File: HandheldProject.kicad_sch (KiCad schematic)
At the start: 16 parts

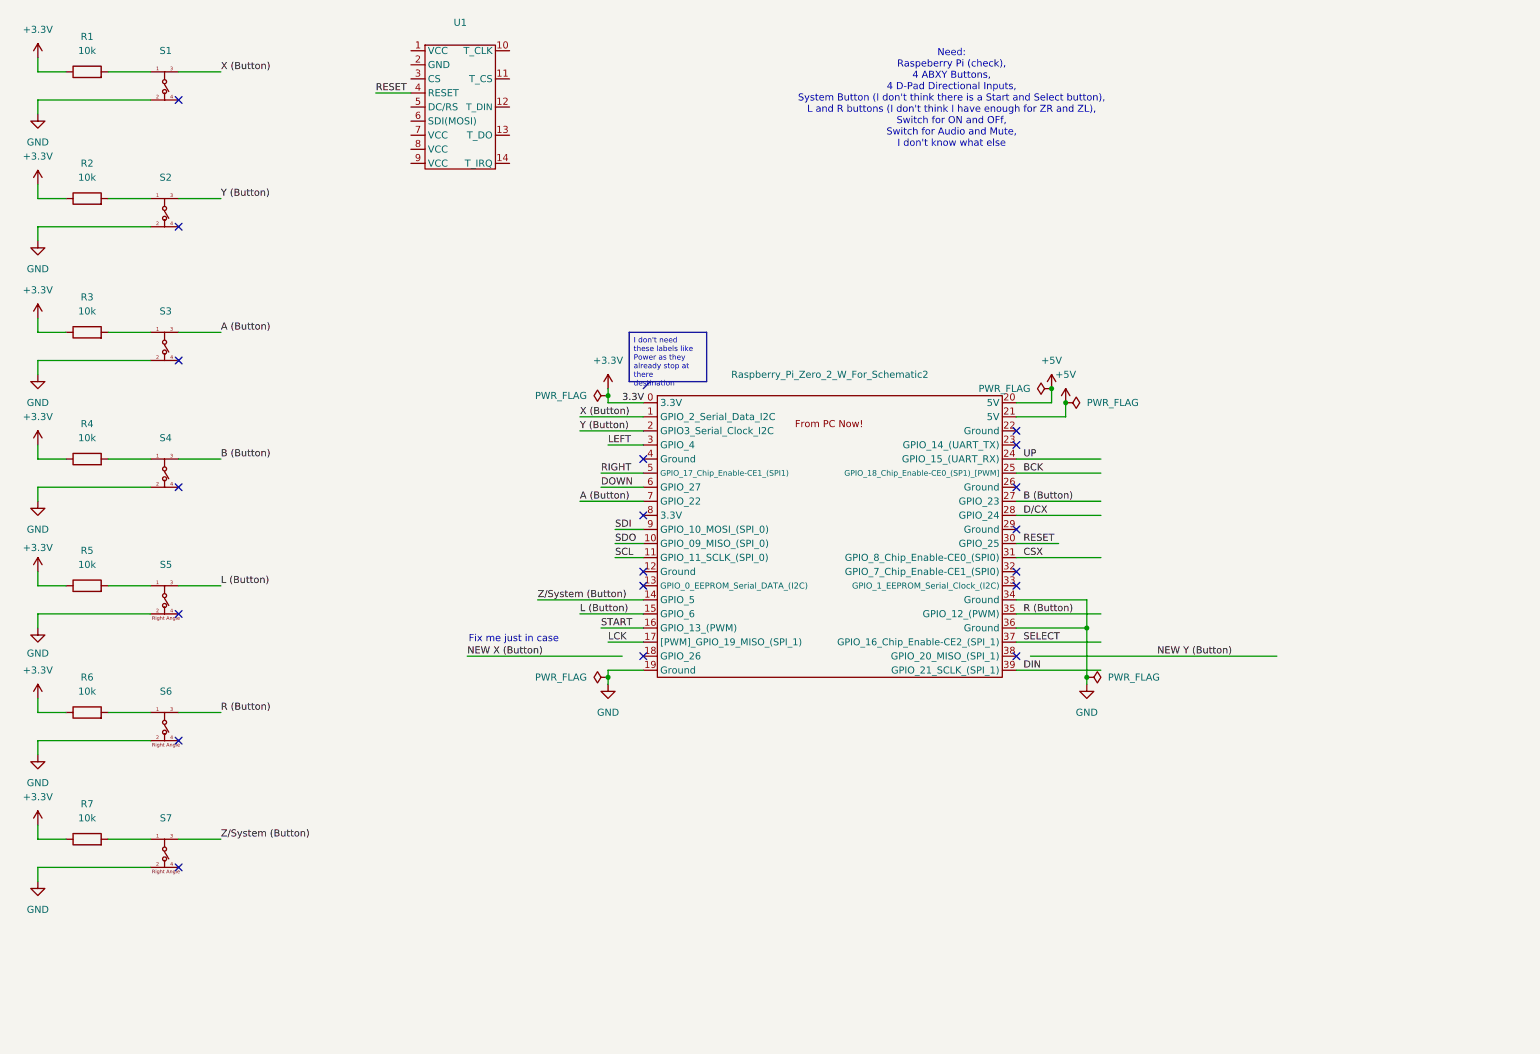
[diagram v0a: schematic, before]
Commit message: Made lots of good work
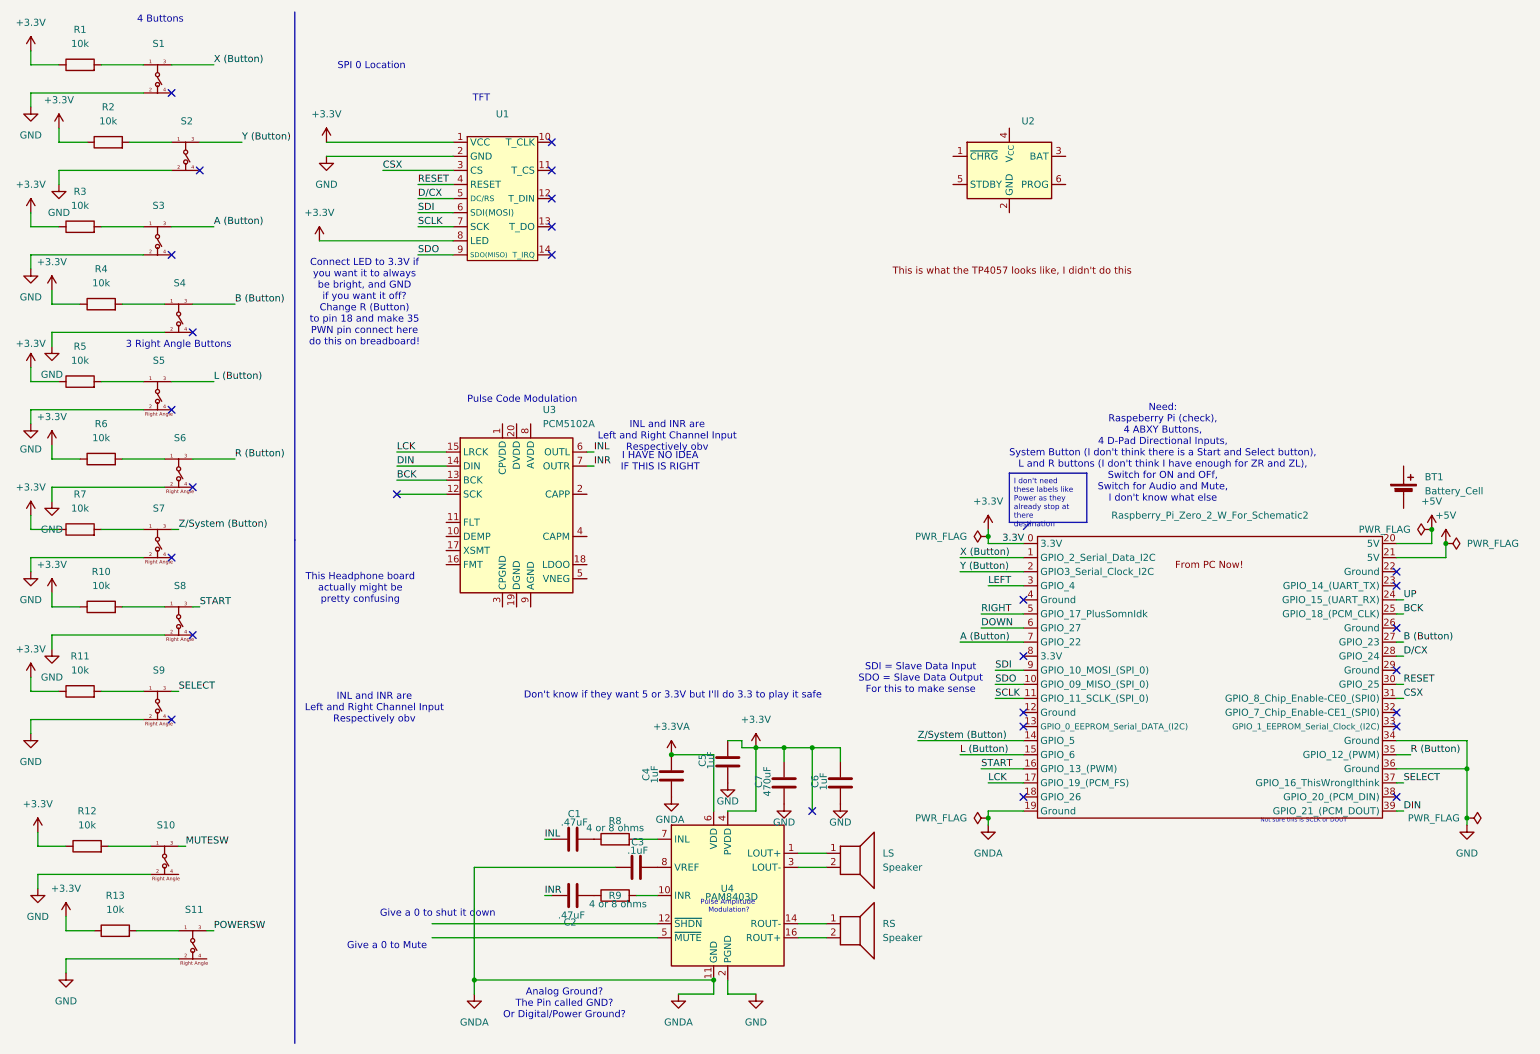
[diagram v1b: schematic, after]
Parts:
- added BT1: Battery_Cell, symbol Device:Battery_Cell
- added C1, C2: .47uF, symbol Device:C
- added C3: .1uF, symbol Device:C
- added C4, C5, C6: 1uF, symbol Device:C
- added C7: 470uF, symbol Device:C
- added LS, RS: Speaker, symbol Device:Speaker
- added R10, R11, R12, R13: 10k, symbol Device:R
- added R8, R9: 4 or 8 ohms, symbol Device:R
- added S10, S11, S8, S9: ~, symbol Shakir_Switch_Library:Right_Angle_Switch
- added U2: ~, symbol Shakir_Handheld_Miscellaneous_Library:TP4056_Battery_Charger
- added U3: PCM5102A, Package_SO:TSSOP-20_4.4x6.5mm_P0.65mm, symbol Audio:PCM5102A
- added U4: PAM8403D, Package_SO:SOP-16_3.9x9.9mm_P1.27mm, symbol Amplifier_Audio:PAM8403D
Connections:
- net SCL is gone; now on net SCLK: Raspberry_Pi_Zero_2_W_For_Schematic2.11 (GPIO_11_SCLK_(SPI_0))
- net +3.3V: now also U1.1 (VCC), U1.8 (LED), C5.2, C6.2, C7.2, R10.1, R11.1, R12.1, R13.1, U4.13 (PVDD), U4.4 (PVDD)
- net BCK: now also U3.13 (BCK)
- net CSX: now also U1.3 (CS)
- net DIN: now also U3.14 (DIN)
- net D/CX: now also U1.5 (DC/RS)
- net GND: now also U1.2 (GND), C5.1, C6.1, C7.1, S10.2, S11.2, S8.2, S9.2, U4.15 (PGND), U4.2 (PGND); no longer Raspberry_Pi_Zero_2_W_For_Schematic2.19 (Ground)
- net LCK: now also U3.15 (LRCK)
- net SDI: now also U1.6 (SDI(MOSI))
- net SDO: now also U1.9 (SDO(MISO))
- net SELECT: now also S9.3
- net START: now also S8.3
- net SCLK: now reaches U1.7 (SCK)
- new net: R13.2, S11.1
- new net: C1.2, R8.1
- new net: R12.2, S10.1
- new net: LS.1, U4.1 (LOUT+)
- new net: LS.2, U4.3 (LOUT-)
- new net: C2.2, R9.1
- new net: RS.1, U4.14 (ROUT-)
- new net: RS.2, U4.16 (ROUT+)
- new net: R9.2, U4.10 (INR)
- new net: R11.2, S9.1
- new net: R8.2, U4.7 (INL)
- new net: C3.2, U4.8 (VREF)
- new net: R10.2, S8.1
- new net +3.3VA: C4.2, U4.6 (VDD)
- new net GNDA: C3.1, C4.1, Raspberry_Pi_Zero_2_W_For_Schematic2.19 (Ground), U4.11 (GND)
- new net INL: C1.1, U3.6 (OUTL)
- new net INR: C2.1, U3.7 (OUTR)
- new net MUTESW: S10.3
- new net POWERSW: S11.3
- no-connect marks 19 -> 28
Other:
- note added: "3 Right Angle Buttons"
- note added: "4 Buttons"
- note added: "Analog Ground? The Pin called GND? Or Digital/Power Ground?"
- note added: "Connect LED to 3.3V if you want it to always be bright, and GND if you want it off? Change R (Button) to pin 18 and make 35 PWN pin connect here do this on breadboard!"
- note added: "Don't know if they want 5 or 3.3V but I'll do 3.3 to play it safe"
- note added: "Give a 0 to Mute"
- note added: "Give a 0 to shut it down"
- note added: "I HAVE NO IDEA IF THIS IS RIGHT"
- note added: "INL and INR are Left and Right Channel Input Respectively obv"
- note added: "Not sure this is SCLK or DOUT"
- note added: "Pulse Amplitude Modulation?"
- note added: "Pulse Code Modulation"
- note added: "SDI = Slave Data Input SDO = Slave Data Output For this to make sense"
- note added: "SPI 0 Location"
- note added: "TFT"
- note added: "This Headphone board actually might be pretty confusing"
- note removed: "Fix me just in case"
- moved on the sheet: R1, R2, R3, R4, R5, R6, R7, Raspberry_Pi_Zero_2_W_For_Schematic2, S1, S2, S3, S4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
